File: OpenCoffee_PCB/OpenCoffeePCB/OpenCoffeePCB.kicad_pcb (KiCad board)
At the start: 2 copper layers, 2 parts, among them U1 Pico, U2 Pico_WiFi

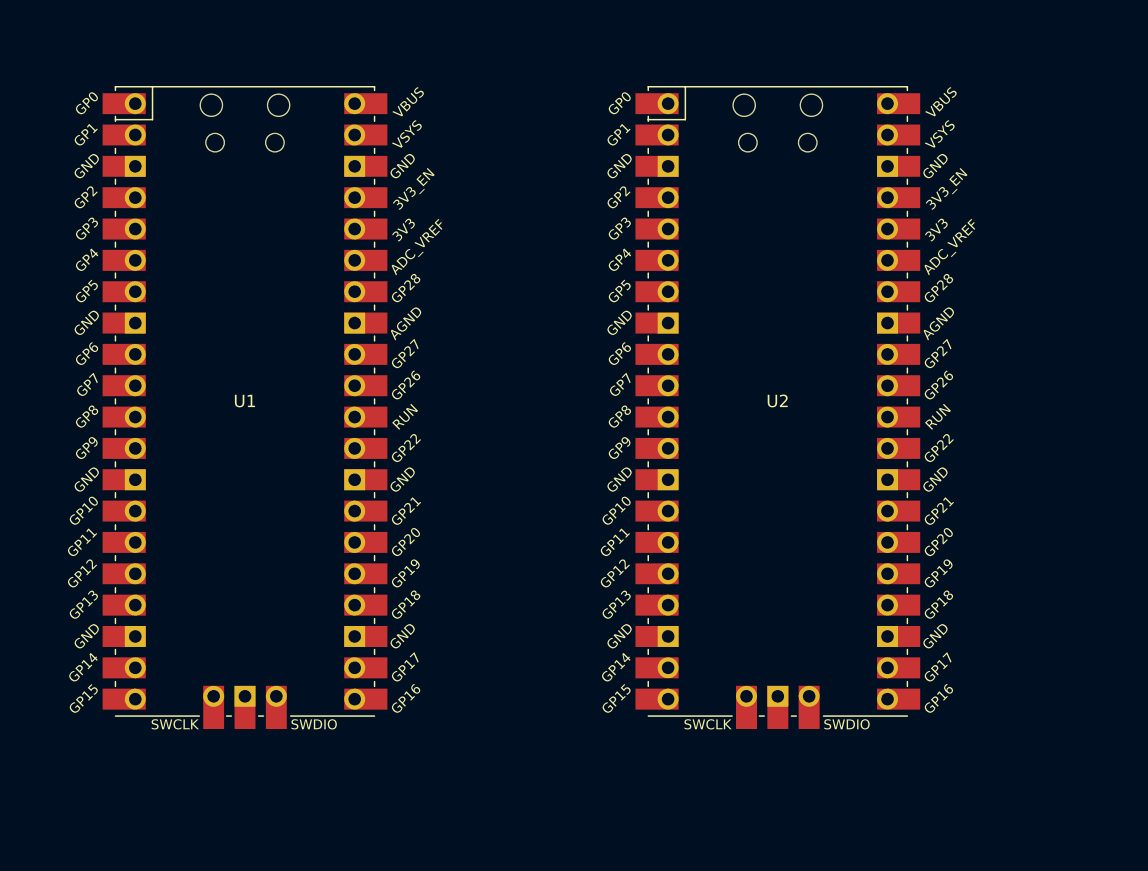
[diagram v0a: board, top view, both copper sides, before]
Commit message: intial layout
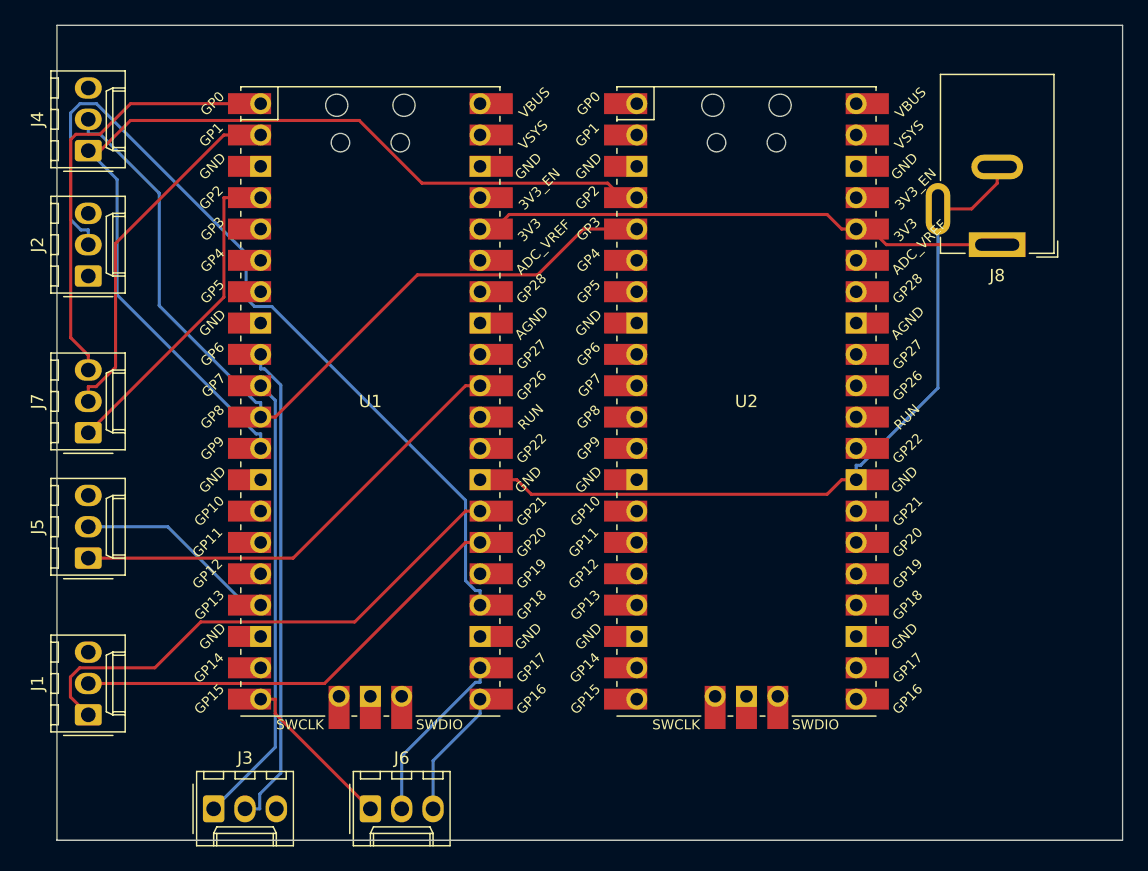
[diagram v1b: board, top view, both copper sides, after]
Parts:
- added J1: Conn_01x02_Male, Connector_Molex:Molex_KK-254_AE-6410-03A_1x03_P2.54mm_Vertical, F.Cu at (111.8, 91.4)
- added J2: Conn_01x02_Male, Connector_Molex:Molex_KK-254_AE-6410-03A_1x03_P2.54mm_Vertical, F.Cu at (111.8, 55.9)
- added J3: Conn_01x02_Male, Connector_Molex:Molex_KK-254_AE-6410-03A_1x03_P2.54mm_Vertical, F.Cu at (121.9, 99.1)
- added J4: Conn_01x02_Male, Connector_Molex:Molex_KK-254_AE-6410-03A_1x03_P2.54mm_Vertical, F.Cu at (111.8, 45.7)
- added J5: Conn_01x02_Male, Connector_Molex:Molex_KK-254_AE-6410-03A_1x03_P2.54mm_Vertical, F.Cu at (111.8, 78.7)
- added J6: Conn_01x03_Male, Connector_Molex:Molex_KK-254_AE-6410-03A_1x03_P2.54mm_Vertical, F.Cu at (134.6, 99.1)
- added J7: Conn_01x03_Male, Connector_Molex:Molex_KK-254_AE-6410-03A_1x03_P2.54mm_Vertical, F.Cu at (111.8, 68.6)
- added J8: Barrel_Jack_Switch, Connector_BarrelJack:BarrelJack_GCT_DCJ200-10-A_Horizontal, F.Cu at (185.4, 53.3)
- moved U1 10.2 mm to (134.6, 66.0)
- moved U2 2.54 mm to (165.1, 66.0)
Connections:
- U1 pad 1: unconnected-(U1-Pad1) -> Rotary_Button
- U1 pad 10: unconnected-(U1-Pad10) -> Display_SCL
- U1 pad 11: unconnected-(U1-Pad11) -> UART_TX
- U1 pad 12: unconnected-(U1-Pad12) -> UART_RX
- U1 pad 17: unconnected-(U1-Pad17) -> GroupHeadSolenoid
- U1 pad 2: unconnected-(U1-Pad2) -> Rotary_DT
- U1 pad 20: unconnected-(U1-Pad20) -> MAX6675_SCK
- U1 pad 21: unconnected-(U1-Pad21) -> MAX6675_CS
- U1 pad 22: unconnected-(U1-Pad22) -> MAX6675_SO
- U1 pad 24: unconnected-(U1-Pad24) -> DimmerPWM
- U1 pad 26: unconnected-(U1-Pad26) -> PressureSDA
- U1 pad 27: unconnected-(U1-Pad27) -> PressureSCL
- U1 pad 28: unconnected-(U1-Pad28) -> GND
- U1 pad 31: unconnected-(U1-Pad31) -> Heater
- U1 pad 36: unconnected-(U1-Pad36) -> 5V
- U1 pad 4: unconnected-(U1-Pad4) -> Rotary_CLK
- U1 pad 9: unconnected-(U1-Pad9) -> Display_SDA
- U2 pad 28: unconnected-(U2-Pad28) -> GND
- U2 pad 36: unconnected-(U2-Pad36) -> 5V
- U2 pad 4: unconnected-(U2-Pad4) -> UART_RX
- U2 pad 5: unconnected-(U2-Pad5) -> UART_TX
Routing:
- net UART_RX: track 0.00 -> 78.2 mm
- net DimmerPWM: track 0.00 -> 68.6 mm
- net UART_TX: track 0.00 -> 67.5 mm
- net GND: track 0.00 -> 63.4 mm
- net 5V: track 0.00 -> 43.4 mm
- net PressureSCL: track 0.00 -> 42.4 mm
- net Display_SDA: track 0.00 -> 39.6 mm
- net Heater: track 0.00 -> 37.5 mm
- net Display_SCL: track 0.00 -> 36.8 mm
- net PressureSDA: track 0.00 -> 36.5 mm
- net Rotary_Button: track 0.00 -> 35.9 mm
- net Rotary_DT: track 0.00 -> 29.5 mm
- net Rotary_CLK: track 0.00 -> 26.6 mm
- net GroupHeadSolenoid: track 0.00 -> 16.6 mm
- net MAX6675_SO: track 0.00 -> 14.3 mm
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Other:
- board outline added: 86.4 x 66 mm
